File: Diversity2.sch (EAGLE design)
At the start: 73 parts, among them IC1 LM1881, IC2 LM1881, IC3 7805TV, IC4 NE5532N, IC5 LM1881, IC6 LM1881, IC7 MEGA16-P, IC9 4052N, Q2 16MHz, U1 AD812ANZ, X1 RCA-4-117-01, X2 RCA-4-117-01, X3 RCA-4-117-01, X4 22-23-2031

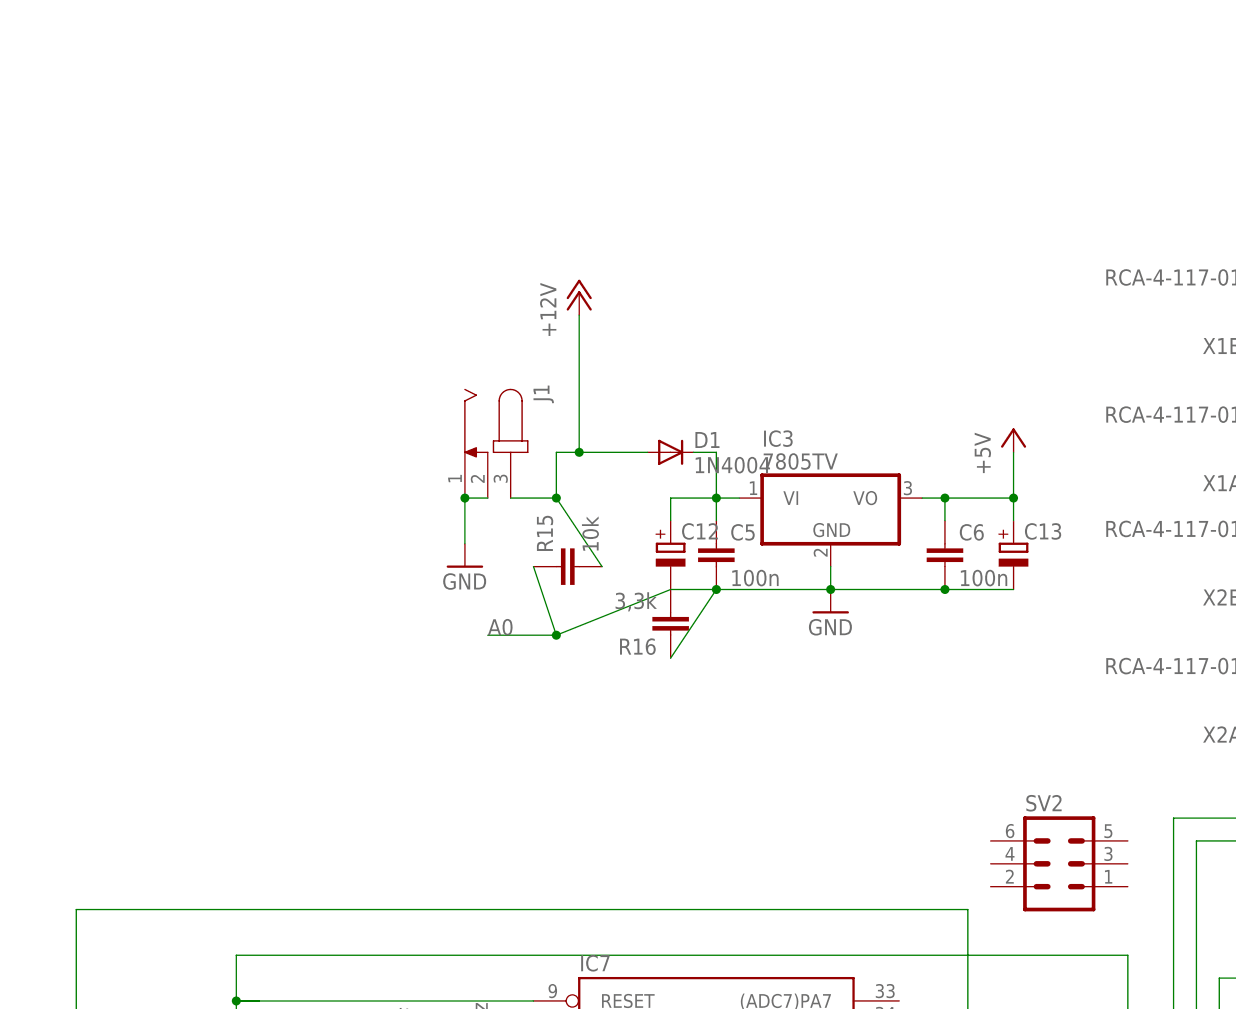
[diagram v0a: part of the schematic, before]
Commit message: asdf
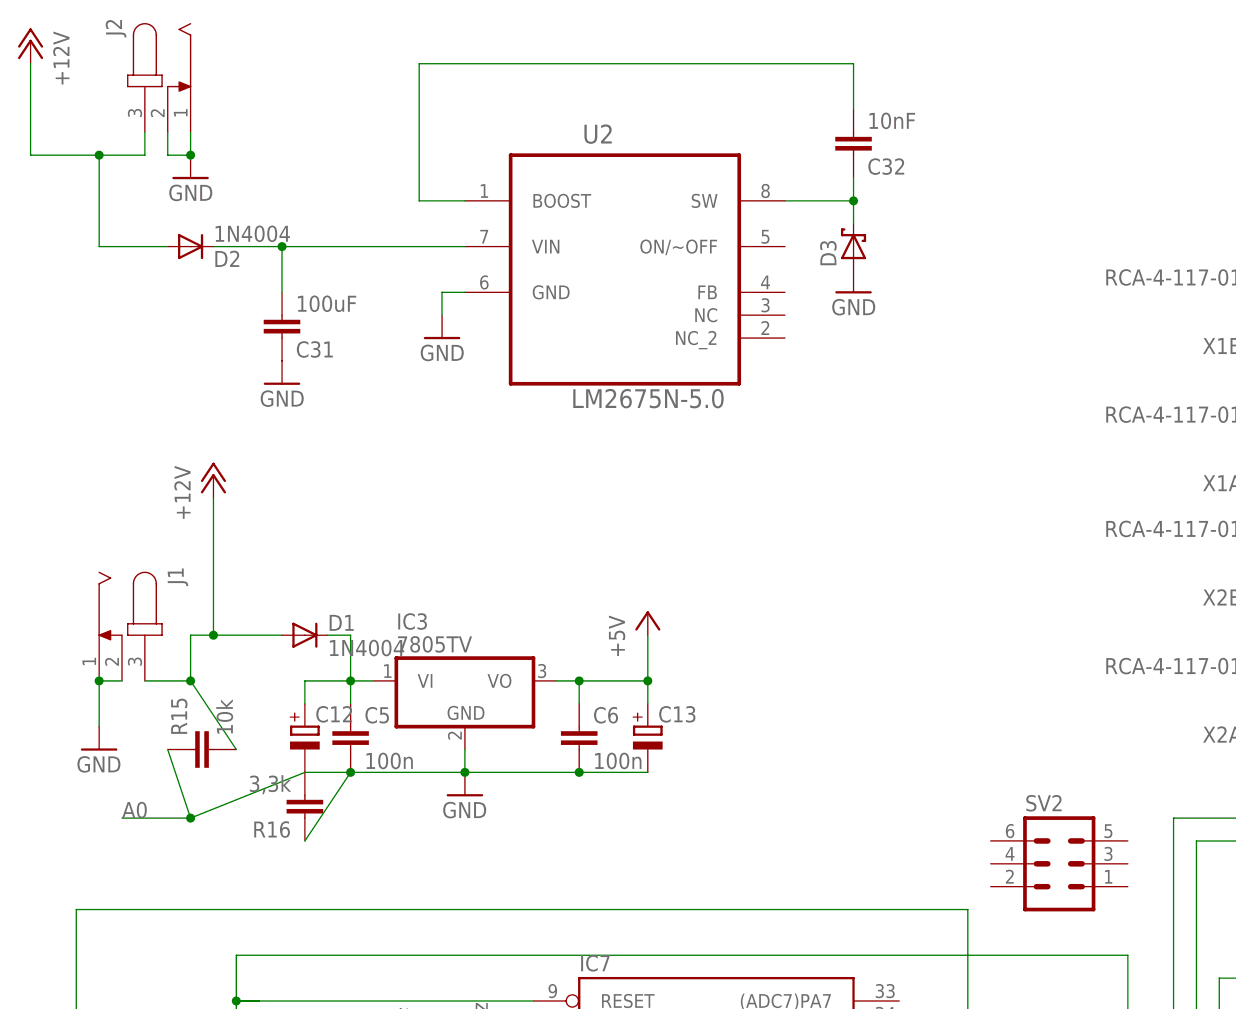
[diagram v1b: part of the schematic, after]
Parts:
- added C31: 100uF, capacitor-wima:C2.5/2
- added C32: 10nF, capacitor-wima:C2.5/2
- added D2: 1N4004, diode:1N4004
- added D3: (no value), diode:SCHOTTKY-DIODECB417-15
- added J2: (no value), con-jack:JACK-PLUG0
- added U2: LM2675N-5.0, NSC_By_element14_Batch_1.1:LM2675N-5.0
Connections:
- new net N$62: C32.2, U2.BOOST
- new net N$63: C31.2, D2.C, U2.VIN
- new net N$64: C32.1, D3.C, U2.SW
- net +12V: now also D2.A, J2.3
- net GND: now also C31.1, D3.A, J2.1, J2.2, U2.GND
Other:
- moved on the sheet: C12, C13, C5, C6, D1, IC3, J1, R15, R16
